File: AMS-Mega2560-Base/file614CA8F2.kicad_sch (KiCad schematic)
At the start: 22 parts, among them IC13 MAX764CPA+, IC14 LM2917N-8_NOPB, J23 Conn_01x02, J24 Conn_01x02, J31 Conn_01x02, K1 DIP05-1A72-12L, Q25 2N7000

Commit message: changing SMD footprint for RPM sensor CAP reDRC'ed and remade the FAB files
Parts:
- C31: footprint Capacitor_Tantalum_SMD:CP_EIA-3528-15_AVX-H_Pad1.50x2.35mm_HandSolder -> Capacitor_SMD:C_0805_2012Metric_Pad1.18x1.45mm_HandSolder
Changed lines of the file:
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@@
       (effects (font (size 1.27 1.27)) (justify left))
     )
-    (property "Footprint" "Capacitor_Tantalum_SMD:CP_EIA-3528-15_AVX-H_Pad1.50x2.35mm_HandSolder" (id 2) (at 153.3652 129.54 0)
+    (property "Footprint" "Capacitor_SMD:C_0805_2012Metric_Pad1.18x1.45mm_HandSolder" (id 2) (at 153.3652 129.54 0)
       (effects (font (size 1.27 1.27)) hide)
     )

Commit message: fixed footprint and synced schem and layout
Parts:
- C32: footprint Capacitor_THT:C_Radial_D4.0mm_H5.0mm_P1.50mm -> Capacitor_THT:CP_Radial_D4.0mm_P1.50mm
- K1: footprint DIP051A7212L -> SamacSys_Parts:DIP051A7212L
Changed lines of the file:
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@@
       (effects (font (size 1.27 1.27)) (justify left))
     )
-    (property "Footprint" "Capacitor_THT:C_Radial_D4.0mm_H5.0mm_P1.50mm" (id 2) (at 166.37 125.73 0)
+    (property "Footprint" "Capacitor_THT:CP_Radial_D4.0mm_P1.50mm" (id 2) (at 166.37 125.73 0)
       (effects (font (size 1.27 1.27)) hide)
     )
@@
     (property "Reference" "K1" (id 0) (at 197.485 64.0293 0))
     (property "Value" "DIP05-1A72-12L" (id 1) (at 197.485 66.8044 0))
-    (property "Footprint" "DIP051A7212L" (id 2) (at 210.185 67.945 0)
+    (property "Footprint" "SamacSys_Parts:DIP051A7212L" (id 2) (at 210.185 67.945 0)
       (effects (font (size 1.27 1.27)) (justify left) hide)
     )

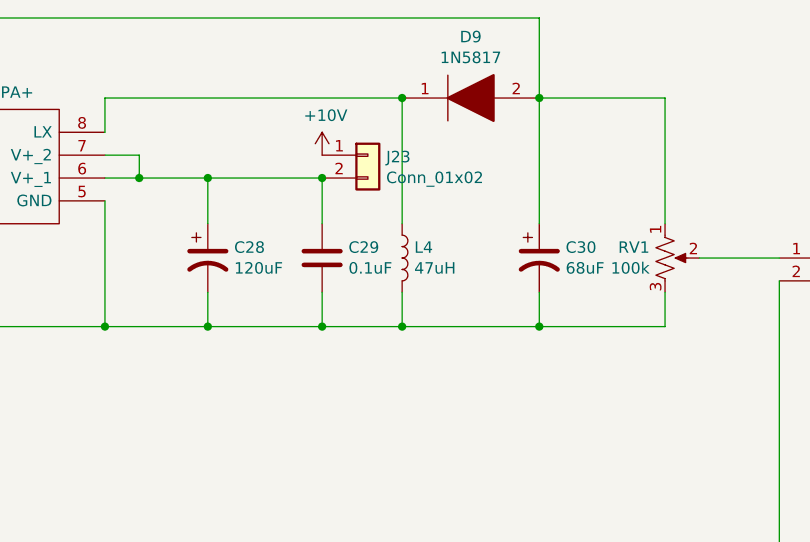
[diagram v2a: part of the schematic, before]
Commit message: working on this.
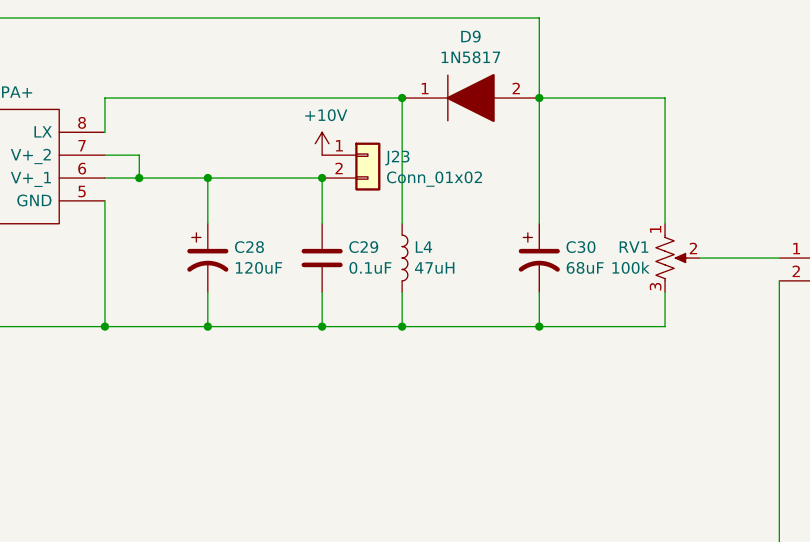
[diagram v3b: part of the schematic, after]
